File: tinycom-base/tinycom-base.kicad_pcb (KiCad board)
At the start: 2 copper layers, 45.2 x 45.2 mm, 10 parts, among them J1 MICRO_SD_HINGE, P1 CONN_02X08, P2 CONN_02X08, P3 USB_A, P4 USB_B, U1 OLIMEX_IC_AXP209

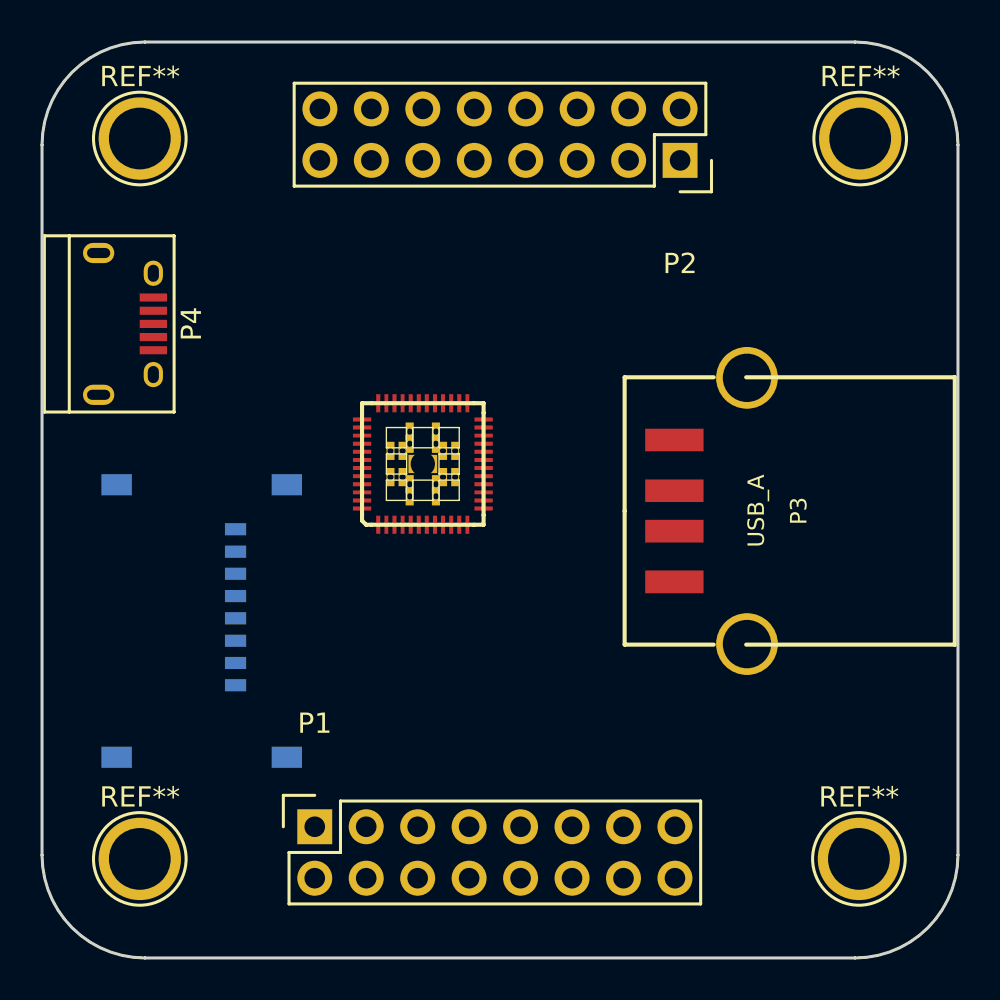
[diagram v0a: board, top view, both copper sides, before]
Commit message: prepare base
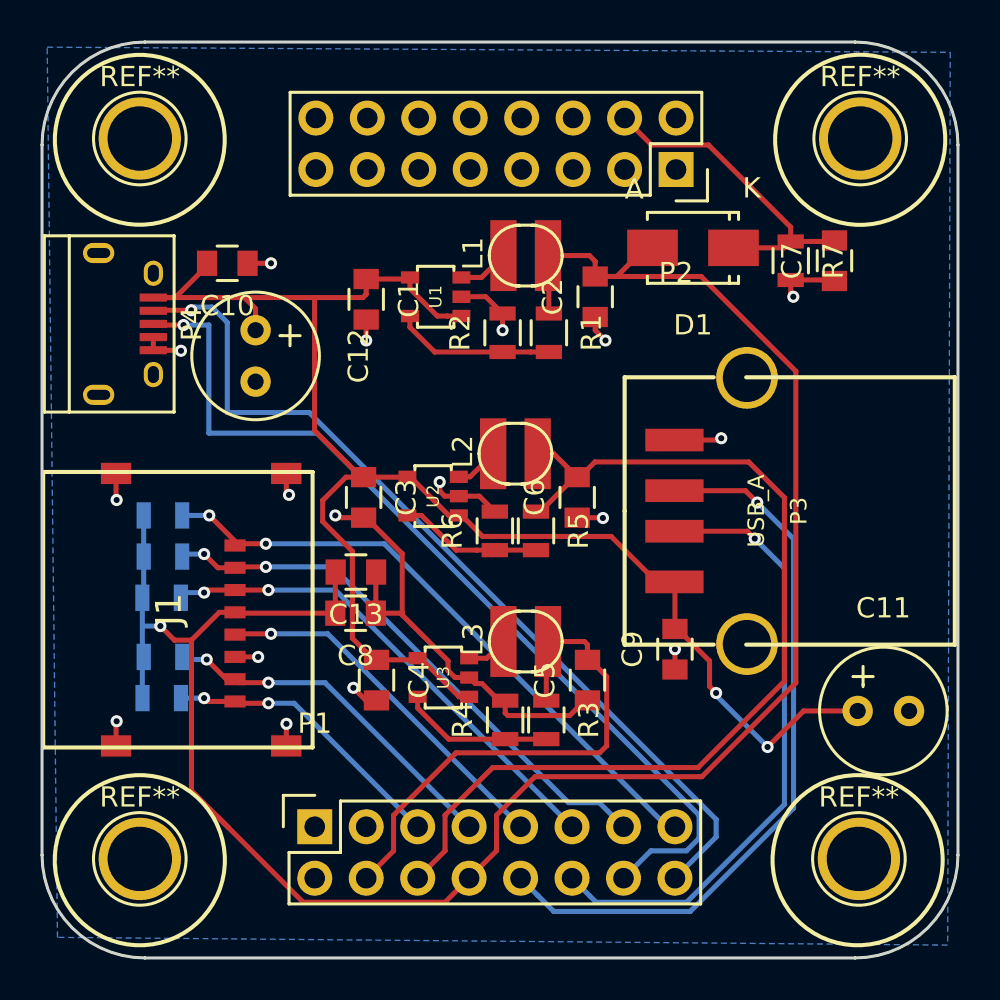
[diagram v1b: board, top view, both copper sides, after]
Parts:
- added C1: C_Small, Capacitors_SMD:C_0805, F.Cu at (140.5, 91.9)
- added C10: C_Small, Capacitors_SMD:C_0805, F.Cu at (133.6, 90.2)
- added C11: CP_Small, Capacitors_Elko_ThroughHole:Elko_vert_11.2x6.3mm_RM2.5_CopperClear, F.Cu at (164.7, 112.3)
- added C12: CP_Small, Capacitors_Elko_ThroughHole:Elko_vert_11.2x6.3mm_RM2.5_CopperClear, F.Cu at (135.0, 93.5)
- added C13: C_Small, Capacitors_SMD:C_0805, F.Cu at (140.0, 105.4)
- added C2: C_Small, Capacitors_SMD:C_0805, F.Cu at (151.8, 91.8)
- added C3: C_Small, Capacitors_SMD:C_0805, F.Cu at (140.3, 101.7)
- added C4: C_Small, Capacitors_SMD:C_0805, F.Cu at (141.0, 110.7)
- added C5: C_Small, Capacitors_SMD:C_0805, F.Cu at (151.4, 110.7)
- added C6: C_Small, Capacitors_SMD:C_0805, F.Cu at (150.9, 101.7)
- added C7: C_Small, Capacitors_SMD:C_0805, F.Cu at (163.6, 90.0)
- added C8: C_Small, Capacitors_SMD:C_0805, F.Cu at (139.9, 107.4)
- added C9: C_Small, Capacitors_SMD:C_0805, F.Cu at (155.7, 109.2)
- added D1: D_Schottky_Small, Diodes_SMD:SMA_Standard, F.Cu at (156.6, 89.4)
- added L1: SMD-INDUCTOR-2.2UH-20%-1.2A(0805), cd32:CD32, F.Cu at (148.3, 89.8)
- added L2: SMD-INDUCTOR-2.2UH-20%-1.2A(0805), cd32:CD32, F.Cu at (147.8, 99.6)
- added L3: SMD-INDUCTOR-2.2UH-20%-1.2A(0805), cd32:CD32, F.Cu at (148.3, 108.8)
- added R1: R_Small, Resistors_SMD:R_0805, F.Cu at (149.5, 93.6)
- added R10: R_Small, Resistors_SMD:R_0805, B.Cu at (130.4, 106.7)
- added R11: R_Small, Resistors_SMD:R_0805, B.Cu at (130.4, 104.6)
- added R12: R_Small, Resistors_SMD:R_0805, B.Cu at (130.4, 102.6)
- added R2: R_Small, Resistors_SMD:R_0805, F.Cu at (147.2, 93.6)
- added R3: R_Small, Resistors_SMD:R_0805, F.Cu at (149.4, 112.7)
- added R4: R_Small, Resistors_SMD:R_0805, F.Cu at (147.3, 112.7)
- added R5: R_Small, Resistors_SMD:R_0805, F.Cu at (148.8, 103.4)
- added R6: R_Small, Resistors_SMD:R_0805, F.Cu at (146.8, 103.4)
- added R7: R_Small, Resistors_SMD:R_0805, F.Cu at (161.4, 90.0)
- added R8: R_Small, Resistors_SMD:R_0805, B.Cu at (130.4, 111.6)
- added R9: R_Small, Resistors_SMD:R_0805, B.Cu at (130.4, 109.6)
- added U2: SY8008BAAC, opendous:SOT23-5_Opendous, F.Cu at (143.8, 101.7)
- added U3: SY8008BAAC, opendous:SOT23-5_Opendous, F.Cu at (144.3, 110.6)
- J1: moved to F.Cu
- U1: value OLIMEX_IC_AXP209 -> SY8008BAAC; footprint tinycom:ax209-OLIMEX_IC_QFN48 -> opendous:SOT23-5_Opendous
- moved U1 8.28 mm to (143.9, 91.8), turned to 90 degrees
- moved J1 0.56 mm to (124.5, 107.3), turned to 90 degrees
- moved P2 0.49 mm to (155.8, 85.5)
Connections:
- net Net-(P1-Pad1) renamed UART1_TX
- net Net-(P1-Pad3) renamed UART1_RX
- J1 pad 1: Net-(J1-Pad1) -> SDC0_D2
- J1 pad 10: Net-(J1-Pad10) -> GND
- J1 pad 11: Net-(J1-Pad11) -> GND
- J1 pad 12: Net-(J1-Pad12) -> GND
- J1 pad 2: Net-(J1-Pad2) -> SDC0_D3
- J1 pad 3: Net-(J1-Pad3) -> SDC0_CMD
- J1 pad 4: Net-(J1-Pad4) -> VCC_33
- J1 pad 5: Net-(J1-Pad5) -> SDC0_CLK
- J1 pad 6: Net-(J1-Pad6) -> GND
- J1 pad 7: Net-(J1-Pad7) -> SDC0_D0
- J1 pad 8: Net-(J1-Pad8) -> SDC0_D1
- J1 pad 9: Net-(J1-Pad9) -> GND
- P1 pad 10: Net-(P1-Pad10) -> UDP1
- P1 pad 11: Net-(P1-Pad11) -> SDC0_CMD
- P1 pad 12: Net-(P1-Pad12) -> UDM1
- P1 pad 13: Net-(P1-Pad13) -> SDC0_D3
- P1 pad 14: Net-(P1-Pad14) -> UDP0
- P1 pad 15: Net-(P1-Pad15) -> SDC0_D2
- P1 pad 16: Net-(P1-Pad16) -> UDM0
- P1 pad 2: Net-(P1-Pad2) -> GND
- P1 pad 4: Net-(P1-Pad4) -> VCC_15
- P1 pad 5: Net-(P1-Pad5) -> SDC0_D1
- P1 pad 6: Net-(P1-Pad6) -> VCC_14
- P1 pad 7: Net-(P1-Pad7) -> SDC0_D0
- P1 pad 8: Net-(P1-Pad8) -> VCC_33
- P1 pad 9: Net-(P1-Pad9) -> SDC0_CLK
- P2 pad 2: Net-(P2-Pad2) -> GND
- P2 pad 4: Net-(P2-Pad4) -> VCC_30
- P3 pad 1: Net-(P3-Pad1) -> +5V
- P3 pad 2: Net-(P3-Pad2) -> UDM1
- P3 pad 3: Net-(P3-Pad3) -> UDP1
- P3 pad 4: Net-(P3-Pad4) -> GND
- P4 pad 1: Net-(P4-Pad1) -> +5V
- P4 pad 2: Net-(P4-Pad2) -> UDM0
- P4 pad 3: Net-(P4-Pad3) -> UDP0
- P4 pad 4: Net-(P4-Pad4) -> GND
- P4 pad 5: Net-(P4-Pad5) -> GND
- U1 pad 1: Net-(U1-Pad1) -> +5V
- U1 pad 2: Net-(U1-Pad2) -> GND
- U1 pad 4: Net-(U1-Pad4) -> +5V
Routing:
- net VCC_33: track 0.00 -> 103.6 mm, vias 0 -> 1
- net +5V: track 0.00 -> 82.2 mm, vias 0 -> 2
- net GND: track 0.00 -> 50.0 mm, vias 0 -> 17
- net VCC_14: track 0.00 -> 48.7 mm
- net UDP0: track 0.00 -> 45.8 mm, vias 0 -> 1
- net UDM0: track 0.00 -> 44.7 mm, vias 0 -> 1
- net UDP1: track 0.00 -> 36.4 mm, vias 0 -> 1
- net SDC0_D2: track 0.00 -> 30.9 mm, vias 0 -> 2
- net UDM1: track 0.00 -> 30.8 mm, vias 0 -> 1
- net SDC0_D3: track 0.00 -> 27.4 mm, vias 0 -> 2
- net VCC_15: track 0.00 -> 26.0 mm
- net SDC0_CMD: track 0.00 -> 24.3 mm, vias 0 -> 2
- net SDC0_CLK: track 0.00 -> 18.1 mm, vias 0 -> 1
- net SDC0_D0: track 0.00 -> 17.6 mm, vias 0 -> 2
- net VCC_30: track 0.00 -> 16.3 mm
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- added copper zone on B.Cu, net GND
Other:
- net class Default: via_drill 0.4 -> 0.3
- rule pad_to_mask_clearance: 0.2 -> 0.07
- board text added: "TinyCom"
- board text added: "http://tinycom.org/"
